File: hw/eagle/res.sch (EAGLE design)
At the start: 63 parts, among them IC2 7805T, IC3 L272M, IC4 L272M, X5 22-23-2021

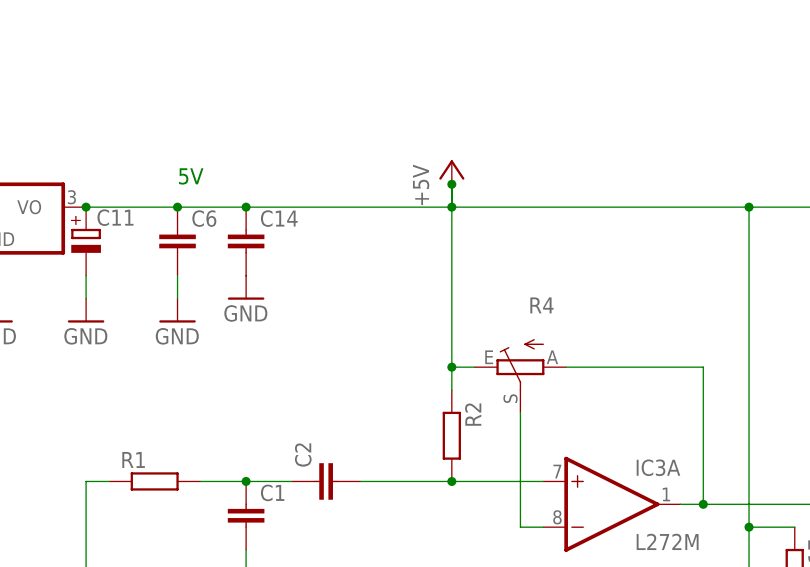
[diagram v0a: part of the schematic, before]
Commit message: +c
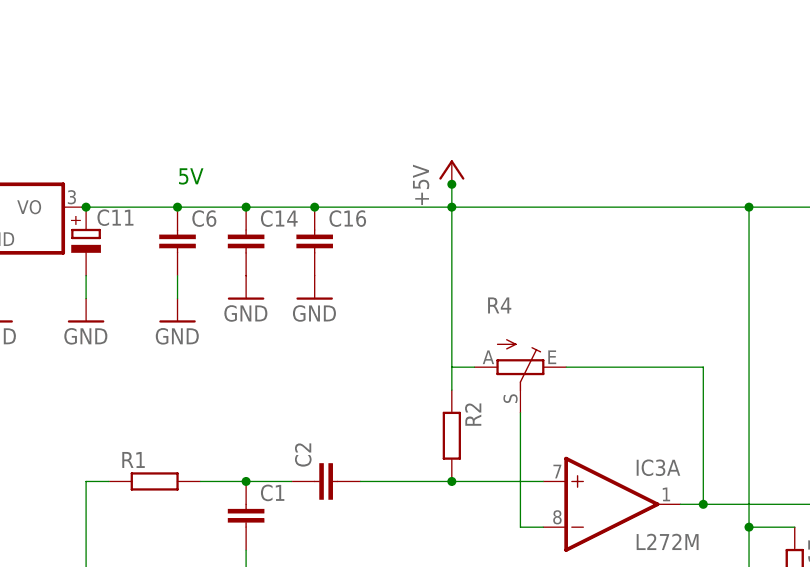
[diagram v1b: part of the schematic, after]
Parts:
- added C16: (no value), rcl:C-EU050-025X075
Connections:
- net +5V: now also C16.1, R4.A; no longer R4.E
- net GND: now also C16.2
- net N$2: now also R4.E; no longer R4.A
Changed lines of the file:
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@@
 <part name="GND35" library="supply1" deviceset="GND" device=""/>
 <part name="GND36" library="supply1" deviceset="GND" device=""/>
+<part name="C16" library="rcl" deviceset="C-EU" device="050-025X075"/>
+<part name="GND37" library="supply1" deviceset="GND" device=""/>
 </parts>
 <sheets>
@@
 <instance part="R2" gate="G$1" x="96.52" y="185.42" rot="R270"/>
 <instance part="R3" gate="G$1" x="152.4" y="177.8" rot="R180"/>
-<instance part="R4" gate="1" x="104.14" y="193.04" rot="MR270"/>
+<instance part="R4" gate="1" x="104.14" y="193.04" rot="R270"/>
 <instance part="R5" gate="G$1" x="144.78" y="200.66" rot="R270"/>
 <instance part="R6" gate="G$1" x="142.24" y="195.58" rot="R270"/>
@@
 <instance part="GND35" gate="1" x="391.16" y="111.76" rot="R90"/>
 <instance part="GND36" gate="1" x="391.16" y="109.22" rot="R90"/>
+<instance part="C16" gate="G$1" x="81.28" y="208.28"/>
+<instance part="GND37" gate="1" x="81.28" y="200.66"/>
 </instances>
 <busses>
@@
 <wire x1="124.46" y1="177.8" x2="121.92" y2="177.8" width="0.1524" layer="91"/>
 <junction x="124.46" y="177.8"/>
-<pinref part="R4" gate="1" pin="A"/>
+<pinref part="R4" gate="1" pin="E"/>
 <wire x1="109.22" y1="193.04" x2="124.46" y2="193.04" width="0.1524" layer="91"/>
 </segment>
@@
 <pinref part="LED2" gate="G$1" pin="C"/>
 <pinref part="GND36" gate="1" pin="GND"/>
+</segment>
+<segment>
+<pinref part="C16" gate="G$1" pin="2"/>
+<pinref part="GND37" gate="1" pin="GND"/>
 </segment>
 </net>
@@
 <segment>
 <pinref part="R2" gate="G$1" pin="1"/>
-<wire x1="96.52" y1="213.36" x2="96.52" y2="210.82" width="0.1524" layer="91"/>
 <wire x1="96.52" y1="210.82" x2="96.52" y2="193.04" width="0.1524" layer="91"/>
 <wire x1="96.52" y1="193.04" x2="96.52" y2="190.5" width="0.1524" layer="91"/>
@@
 <wire x1="142.24" y1="210.82" x2="129.54" y2="210.82" width="0.1524" layer="91"/>
 <wire x1="129.54" y1="210.82" x2="96.52" y2="210.82" width="0.1524" layer="91"/>
-<wire x1="96.52" y1="210.82" x2="73.66" y2="210.82" width="0.1524" layer="91"/>
+<wire x1="96.52" y1="210.82" x2="81.28" y2="210.82" width="0.1524" layer="91"/>
+<wire x1="81.28" y1="210.82" x2="73.66" y2="210.82" width="0.1524" layer="91"/>
 <wire x1="73.66" y1="210.82" x2="66.04" y2="210.82" width="0.1524" layer="91"/>
 <wire x1="96.52" y1="213.36" x2="96.52" y2="210.82" width="0.1524" layer="91"/>
@@
 <junction x="66.04" y="210.82"/>
 <junction x="129.54" y="210.82"/>
-<pinref part="R4" gate="1" pin="E"/>
 <wire x1="129.54" y1="175.26" x2="129.54" y2="210.82" width="0.1524" layer="91"/>
-<wire x1="96.52" y1="193.04" x2="99.06" y2="193.04" width="0.1524" layer="91"/>
 <pinref part="X1" gate="-" pin="3"/>
 <wire x1="160.02" y1="190.5" x2="152.4" y2="190.5" width="0.1524" layer="91"/>
@@
 <junction x="73.66" y="210.82"/>
 <junction x="96.52" y="210.82"/>
-<junction x="96.52" y="193.04"/>
 <junction x="152.4" y="220.98"/>
 <junction x="129.54" y="175.26"/>
-</segment>
-<segment>
+<pinref part="R4" gate="1" pin="A"/>
+<wire x1="96.52" y1="193.04" x2="99.06" y2="193.04" width="0.1524" layer="91"/>
+<pinref part="C16" gate="G$1" pin="1"/>
+<junction x="81.28" y="210.82"/>
+</segment>
+<segment>

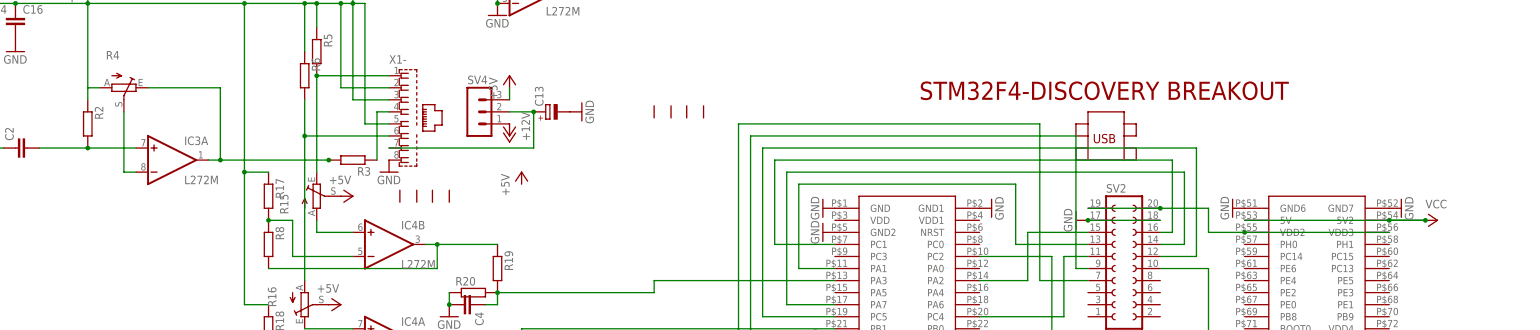
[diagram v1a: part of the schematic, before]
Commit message: gnd
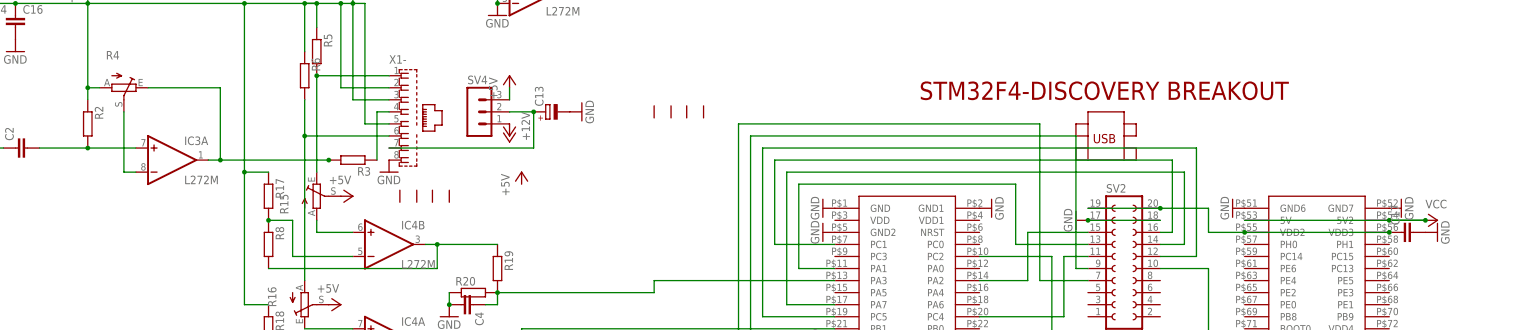
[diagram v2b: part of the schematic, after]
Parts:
- added C17: (no value), rcl:C-EU050-025X075
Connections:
- net GND: now also C17.2
- net N$36: now also C17.1
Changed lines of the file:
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@@
 <part name="C16" library="rcl" deviceset="C-EU" device="050-025X075"/>
 <part name="GND37" library="supply1" deviceset="GND" device=""/>
+<part name="C17" library="rcl" deviceset="C-EU" device="050-025X075"/>
+<part name="GND38" library="supply1" deviceset="GND" device=""/>
 </parts>
 <sheets>
@@
 <instance part="C16" gate="G$1" x="81.28" y="208.28"/>
 <instance part="GND37" gate="1" x="81.28" y="200.66"/>
+<instance part="C17" gate="G$1" x="373.38" y="162.56" rot="R90"/>
+<instance part="GND38" gate="1" x="381" y="162.56" rot="R90"/>
 </instances>
 <busses>
@@
 <pinref part="GND37" gate="1" pin="GND"/>
 </segment>
+<segment>
+<pinref part="C17" gate="G$1" pin="2"/>
+<pinref part="GND38" gate="1" pin="GND"/>
+</segment>
 </net>
 <net name="N$8" class="0">
@@
 <junction x="322.58" y="167.64"/>
 <junction x="340.36" y="162.56"/>
+<pinref part="C17" gate="G$1" pin="1"/>
+<junction x="370.84" y="162.56"/>
 </segment>
 </net>
@@
 <pinref part="C16" gate="G$1" pin="1"/>
 <junction x="81.28" y="210.82"/>
-</segment>
-<segment>
+<junction x="96.52" y="193.04"/>
+</segment>
+<segment>
